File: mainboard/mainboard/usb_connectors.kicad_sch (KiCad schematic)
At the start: 39 parts, among them U7 SY6280, U8 GL852, Y2 ABLS-12.000MHZ-B4-T

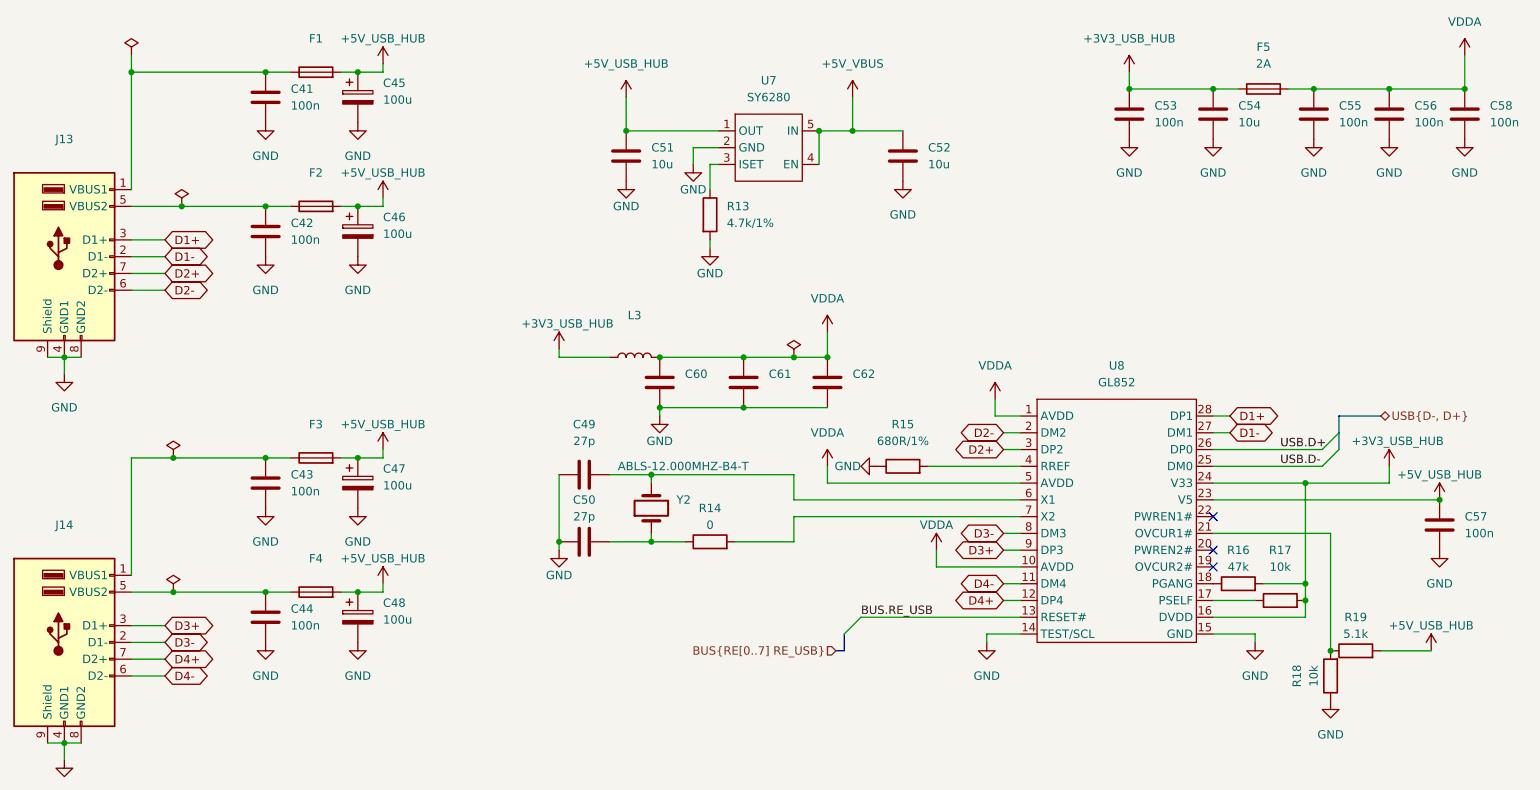
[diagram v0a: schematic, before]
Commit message: board almost ready, paths must be aligned
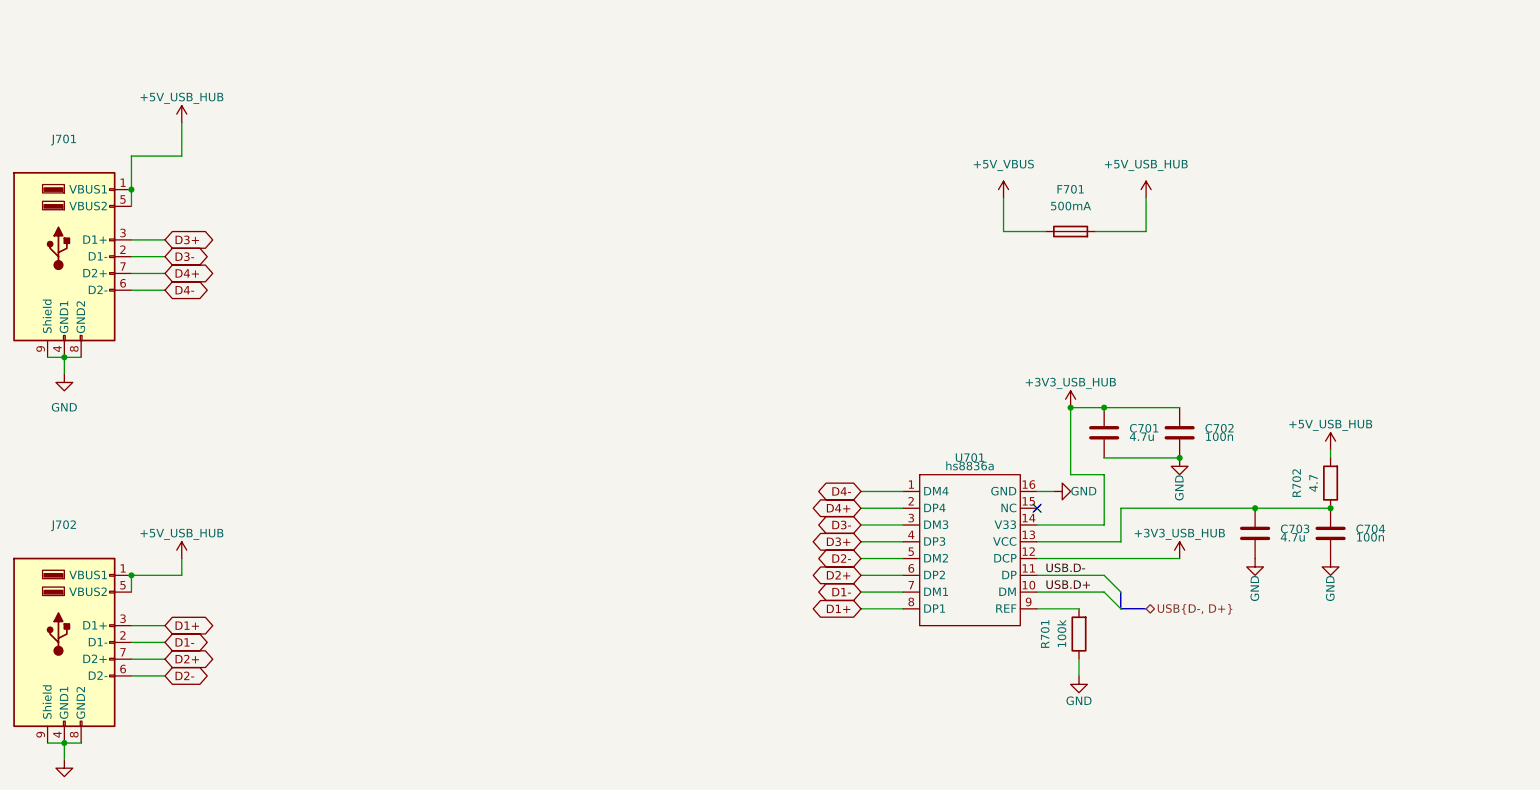
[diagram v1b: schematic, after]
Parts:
- removed C41, C42, C43, C44, C53, C55, C56, C57, C58: 100n, symbol Device:C
- removed C45, C46, C47, C48: 100u, symbol Device:C_Polarized
- removed C49, C50: 27p, Capacitor_SMD:C_0402_1005Metric_Pad0.74x0.62mm_HandSolder, symbol Device:C
- removed C51, C52, C54: 10u, symbol Device:C
- removed C60, C61, C62: (no value), symbol Device:C
- removed F1, F2, F3, F4: (no value), symbol Device:Fuse
- removed F5: 2A, symbol Device:Fuse
- removed L3: (no value), symbol Device:L
- removed R13: 4.7k/1%, symbol Device:R
- removed R14: 0, Resistor_SMD:R_0402_1005Metric_Pad0.72x0.64mm_HandSolder, symbol Device:R
- removed R15: 680R/1%, symbol Device:R
- removed R16: 47k, symbol Device:R
- removed R17, R18: 10k, symbol Device:R
- removed R19: 5.1k, symbol Device:R
- removed U7: SY6280, Package_TO_SOT_SMD:SOT-23-5_HandSoldering, symbol project_power:SY6280
- removed U8: GL852, Package_SO:SSOP-28_5.3x10.2mm_P0.65mm, symbol Genesys:GL852
- removed Y2: ABLS-12.000MHZ-B4-T, Crystal:Crystal_SMD_HC49-SD_HandSoldering, symbol Device:Crystal
- added C701, C703: 4.7u, Capacitor_SMD:C_0603_1608Metric_Pad1.08x0.95mm_HandSolder, symbol Device:C
- added C702, C704: 100n, Capacitor_SMD:C_0603_1608Metric_Pad1.08x0.95mm_HandSolder, symbol Device:C
- added F701: 500mA, Fuse:Fuse_1206_3216Metric_Pad1.42x1.75mm_HandSolder, symbol Device:Fuse
- added R701: 100k, Resistor_SMD:R_0603_1608Metric_Pad0.98x0.95mm_HandSolder, symbol Device:R
- added R702: 4.7, Resistor_SMD:R_0603_1608Metric_Pad0.98x0.95mm_HandSolder, symbol Device:R
- added U701: hs8836a, Package_SO:SOP-16_3.9x9.9mm_P1.27mm, symbol HS8836A:hs8836a
- J701: renamed from J13; footprint (none) -> Connector_USB:USB_A_Wuerth_61400826021_Horizontal_Stacked
- J702: renamed from J14; footprint (none) -> Connector_USB:USB_A_Wuerth_61400826021_Horizontal_Stacked
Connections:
- net +5V_USB_HUB: now also J701.1 (VBUS1), J701.5 (VBUS2), J702.1 (VBUS1), J702.5 (VBUS2), F701.2, R702.2
- net +5V_VBUS: now also F701.1
- net D1+: now also J702.3 (D1+), U701.8 (DP1); no longer J701.3 (D1+)
- net D1-: now also J702.2 (D1-), U701.7 (DM1); no longer J701.2 (D1-)
- net D2+: now also J702.7 (D2+), U701.6 (DP2); no longer J701.7 (D2+)
- net D2-: now also J702.6 (D2-), U701.5 (DM2); no longer J701.6 (D2-)
- net D3+: now also J701.3 (D1+), U701.4 (DP3); no longer J702.3 (D1+)
- net D3-: now also J701.2 (D1-), U701.3 (DM3); no longer J702.2 (D1-)
- net D4+: now also J701.7 (D2+), U701.2 (DP4); no longer J702.7 (D2+)
- net D4-: now also J701.6 (D2-), U701.1 (DM4); no longer J702.6 (D2-)
- net GND: now also C701.2, C702.2, C703.2, C704.2, R701.1, U701.16 (GND)
- net USB.D+: now also U701.10 (DM)
- net USB.D-: now also U701.11 (DP)
- new net: C703.1, C704.1, R702.1, U701.13 (VCC)
- new net: R701.2, U701.9 (REF)
- new net +3V3_USB_HUB: C701.1, C702.1, U701.12 (DCP), U701.14 (V33)
- no-connect marks 3 -> 1
